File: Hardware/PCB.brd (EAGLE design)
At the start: 46 x 35 mm, 105 parts, among them IC1 BQ25180YBGR_BQ25180YBGR, IC3 BMA421, IC4 DRV2605YZFR, IC9 RT6160AWSC, J1 503480-2400, J2 TC2030-IDC, J4 KH-TYPE-C-16P, Q1 20V/4.2A/52mΩ/1.4W, Q3 SI1308EDL-T1-GE3, U1 NRF52840_QF, U3 MAX17048G+T10, X1 32MHz, X2 32.768kHz

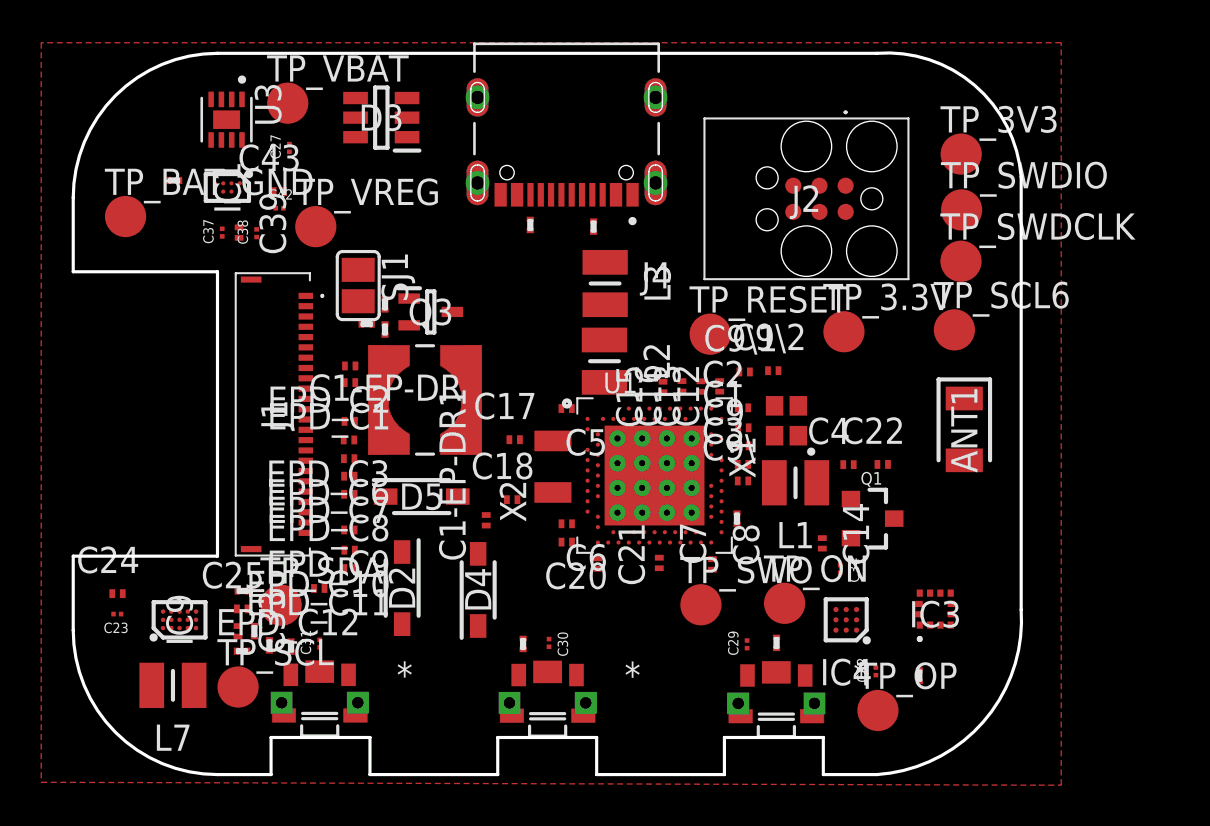
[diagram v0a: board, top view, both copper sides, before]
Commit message: Final Project
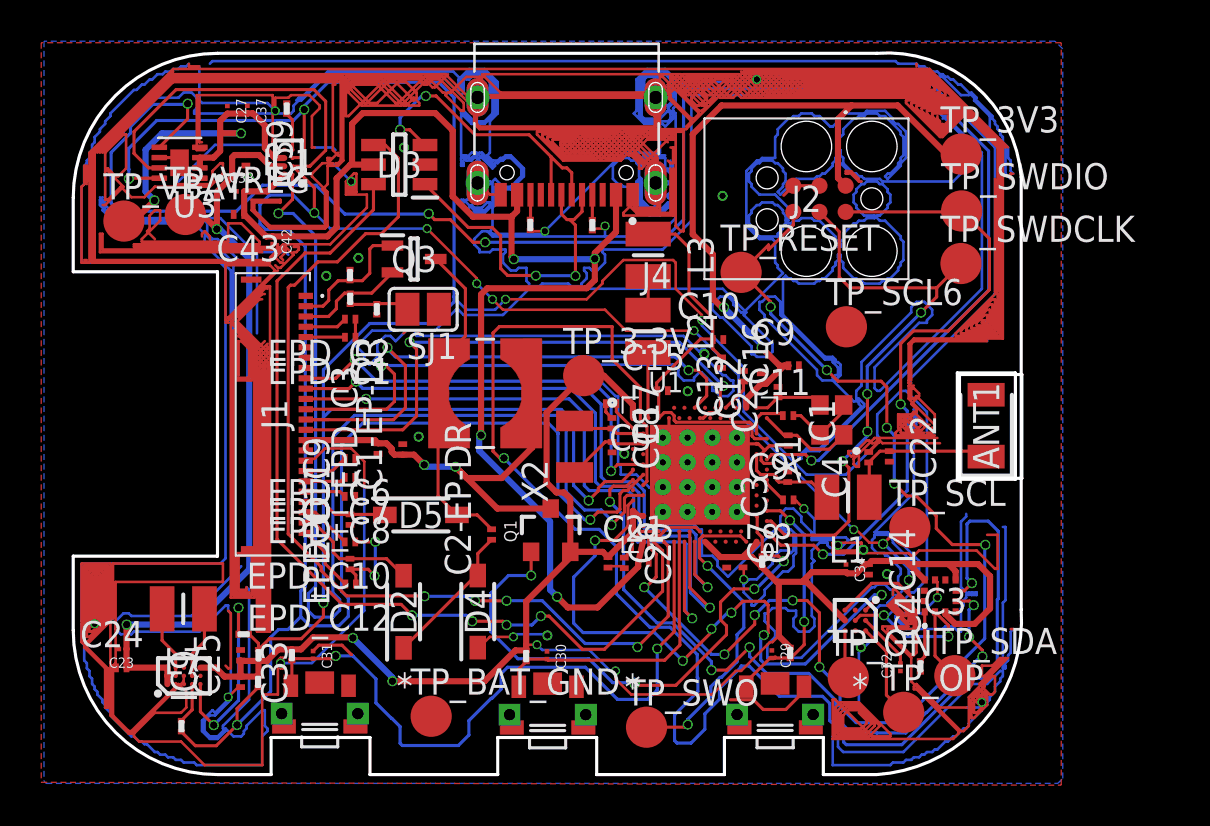
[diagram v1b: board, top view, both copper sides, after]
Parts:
- removed C1-EP-DR1: 22uF, InkTime_v5:NORDIC_NRF_3_RESC0201_L
- removed C9\1, C9\2: 820pF, InkTime_v5:NORDIC_NRF_3_RESC0201_L
- added C10: N.C., InkTime_v5:NORDIC_NRF_3_RESC0201_L
- added C11: 100pF, InkTime_v5:NORDIC_NRF_3_RESC0201_L
- added C2-EP-DR: 4.7uF/25V, InkTime_v5:NORDIC_NRF_3_RESC0201_L
- C1-EP-DR: value 22uF -> 10uF
- moved TP_SCL 33.5 mm to (17.1, -5.36)
- moved TP_SDA 32.9 mm to (19.3, -12.6)
- moved TP_BAT_GND 28.4 mm to (-6.15, -14.5)
- moved Q1 15.6 mm to (-0.35, -5.54), turned to 0 degrees
- moved TP_3.3V 12.8 mm to (1.25, 2.01)
- moved TP_VBAT 9.79 mm to (-21.1, 9.51)
- moved TP_SWO 6.50 mm to (4.30, -15.1)
- moved R1 6.49 mm to (-13.2, 15.0), turned to 0 degrees
- moved TP_VREG 6.36 mm to (-18.1, 9.83)
- moved C37 6.09 mm to (-15.1, 14.9), turned to 270 degrees
- moved C18 5.48 mm to (2.63, -1.46), turned to 270 degrees
- moved TP_SCL6 5.24 mm to (14.0, 4.38)
- moved C17 4.79 mm to (2.62, -0.30), turned to 270 degrees
- moved TP_ON 4.74 mm to (14.1, -12.6)
- moved R4 4.68 mm to (-18.3, -15.0), turned to 0 degrees
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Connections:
- removed net SDA/1.4C: IC4.B2
- net DEC3: now also C11.1; no longer C9\1.1
- net DEC4_6: now also C10.1; no longer C9\2.1
- net GND: now also C10.2, C11.2; no longer C9\1.2, C9\2.2
- net N$14: now also C2-EP-DR.2; no longer C1-EP-DR1.2
- net N$15: now also C2-EP-DR.1; no longer C1-EP-DR1.1
- net SDA: now also IC4.B2
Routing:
- net GND: track 0.00 -> 2060.6 mm, vias 0 -> 29
- net SCL: track 0.00 -> 133.4 mm, vias 0 -> 10
- net SDA: track 0.00 -> 132.2 mm, vias 0 -> 8
- net 3V3: track 0.00 -> 125.2 mm, vias 0 -> 6
- net ALERT: track 0.00 -> 83.5 mm, vias 0 -> 4
- net IMU_INT2: track 0.00 -> 74.2 mm, vias 0 -> 2
- net VBUS: track 0.00 -> 67.0 mm, vias 0 -> 4
- net RESET: track 0.00 -> 60.6 mm, vias 0 -> 10
- net PMIC_INT: track 0.00 -> 53.8 mm, vias 0 -> 2
- net D+: track 0.00 -> 48.2 mm, vias 0 -> 4
- net D-: track 0.00 -> 44.9 mm, vias 0 -> 4
- net VREG: track 0.00 -> 37.6 mm, vias 0 -> 2
- net IMU_INT1: track 0.00 -> 34.0 mm, vias 0 -> 6
- net EPD_RST: track 0.00 -> 33.1 mm, vias 0 -> 2
- net P0.13: track 0.00 -> 32.8 mm, vias 0 -> 2
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- added copper zone on layer 16, net GND
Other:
- outline, holes or cut-outs redrawn
